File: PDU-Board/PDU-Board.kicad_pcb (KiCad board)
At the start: 2 copper layers, 210 x 93 mm, 15 parts, among them J0 Main Feed, J1 Motor-1, J2 Motor-2, J3 Mother Board, J4 RJ45, U1 VICOR-DC-DC, U2 VICOR-DC-DC, U3 VICOR-DC-DC, U4 VICOR-DC-DC, U5 ESC:TMP235A2DBZT, U6 ESC:TMP235A2DBZT

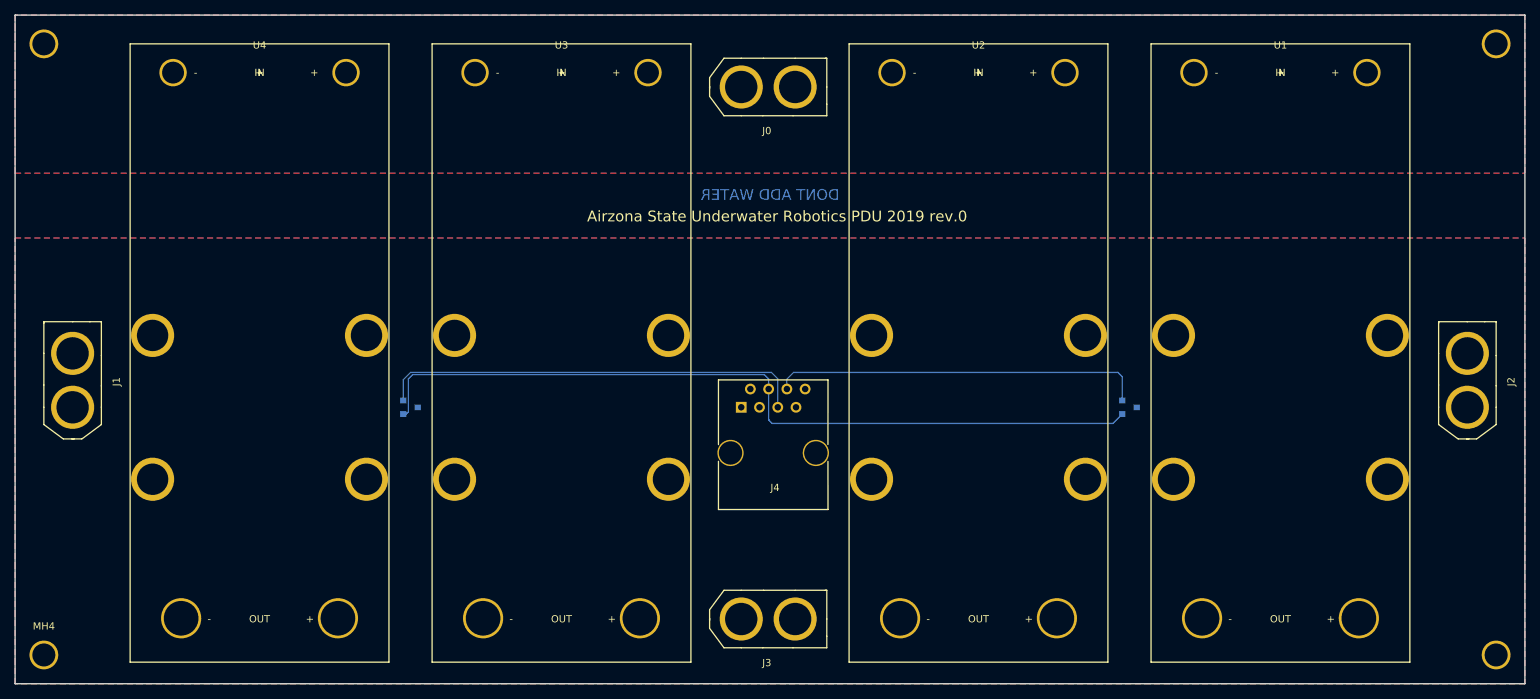
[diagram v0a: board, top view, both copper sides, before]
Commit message: Re designed PDU pre mec spec
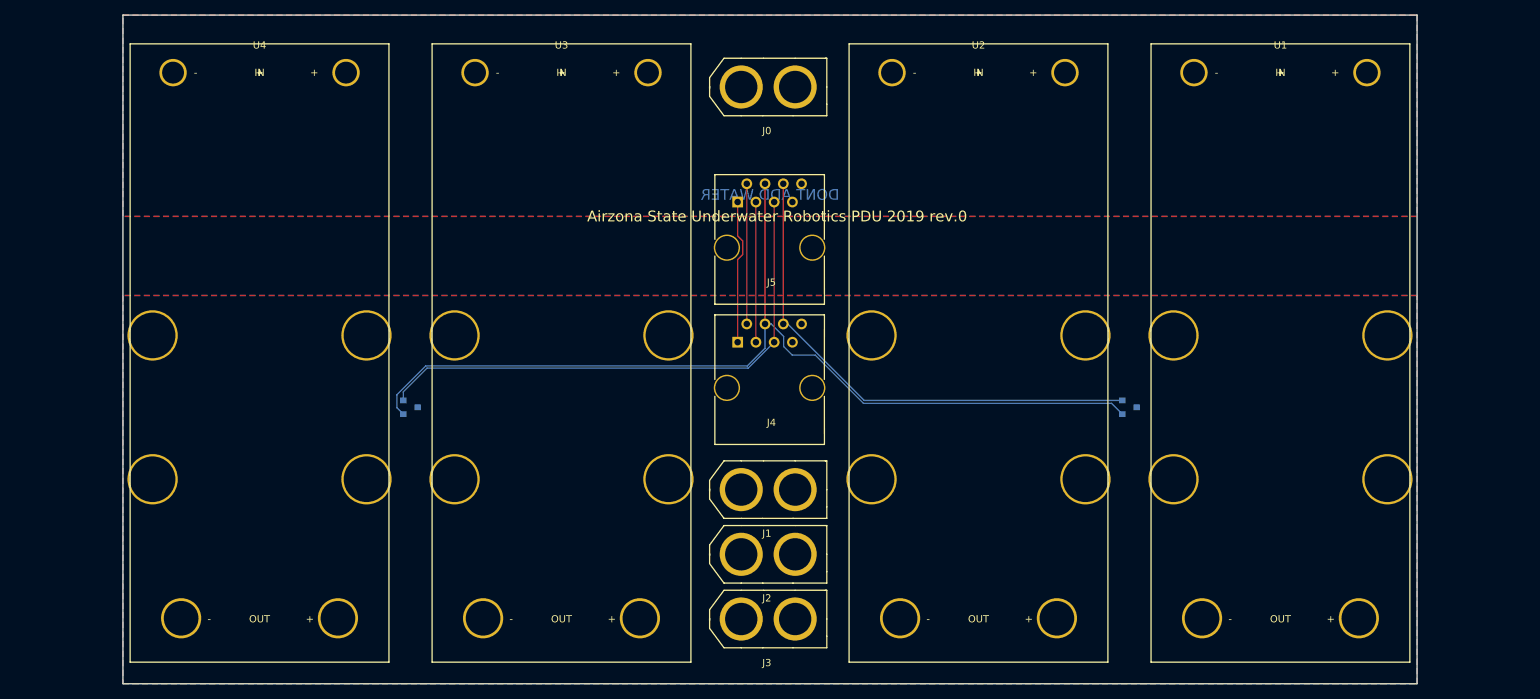
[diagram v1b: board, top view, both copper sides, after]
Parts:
- removed MH1, MH2, MH3, MH4: MountingHole, Blue_ESC:MountingHole_3mm_custom
- added J5: RJ45, Connectors:RJ45_8, F.Cu at (180.5, 106.0)
- moved J2 103.0 mm to (181.0, 155.0), turned to 0 degrees
- moved J1 93.7 mm to (181.0, 146.0), turned to 0 degrees
- moved J4 9.06 mm to (180.5, 125.5)
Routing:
- net +3V3: track 111.7 -> 135.5 mm
- net Net-(J4-Pad1): track 0.00 -> 20.1 mm
- net Net-(J4-Pad2): track 0.00 -> 19.5 mm
- net GND: track 0.00 -> 19.5 mm
- net Ext_Temp_1: track 52.0 -> 70.4 mm
- net Ext_Temp_0: track 59.7 -> 75.1 mm
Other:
- board size 210 x 93 mm -> 180 x 93 mm
